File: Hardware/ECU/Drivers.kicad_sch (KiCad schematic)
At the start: 52 parts, among them SW4 SW_DPDT_x2, U10 TC4424A, U5 TC4424A, U6 TC4424A, U7 MC33810, U8 MC33810, U9 TC4424A

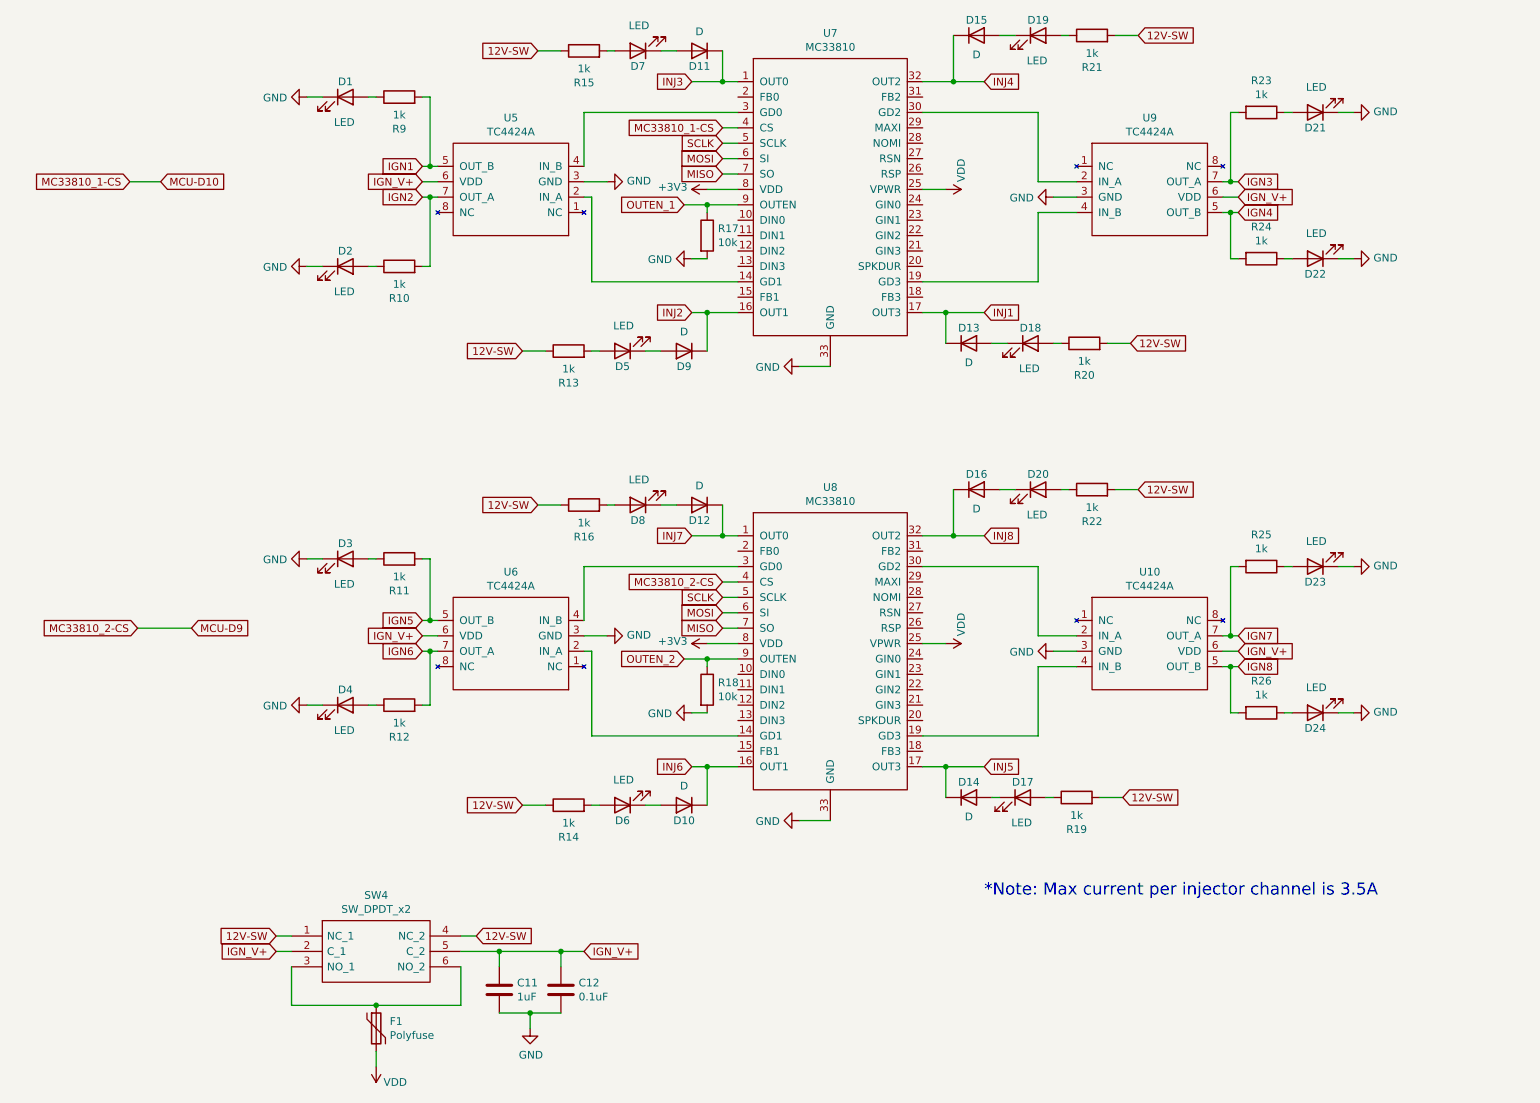
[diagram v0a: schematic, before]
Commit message: PCB
Platine Vernetzt
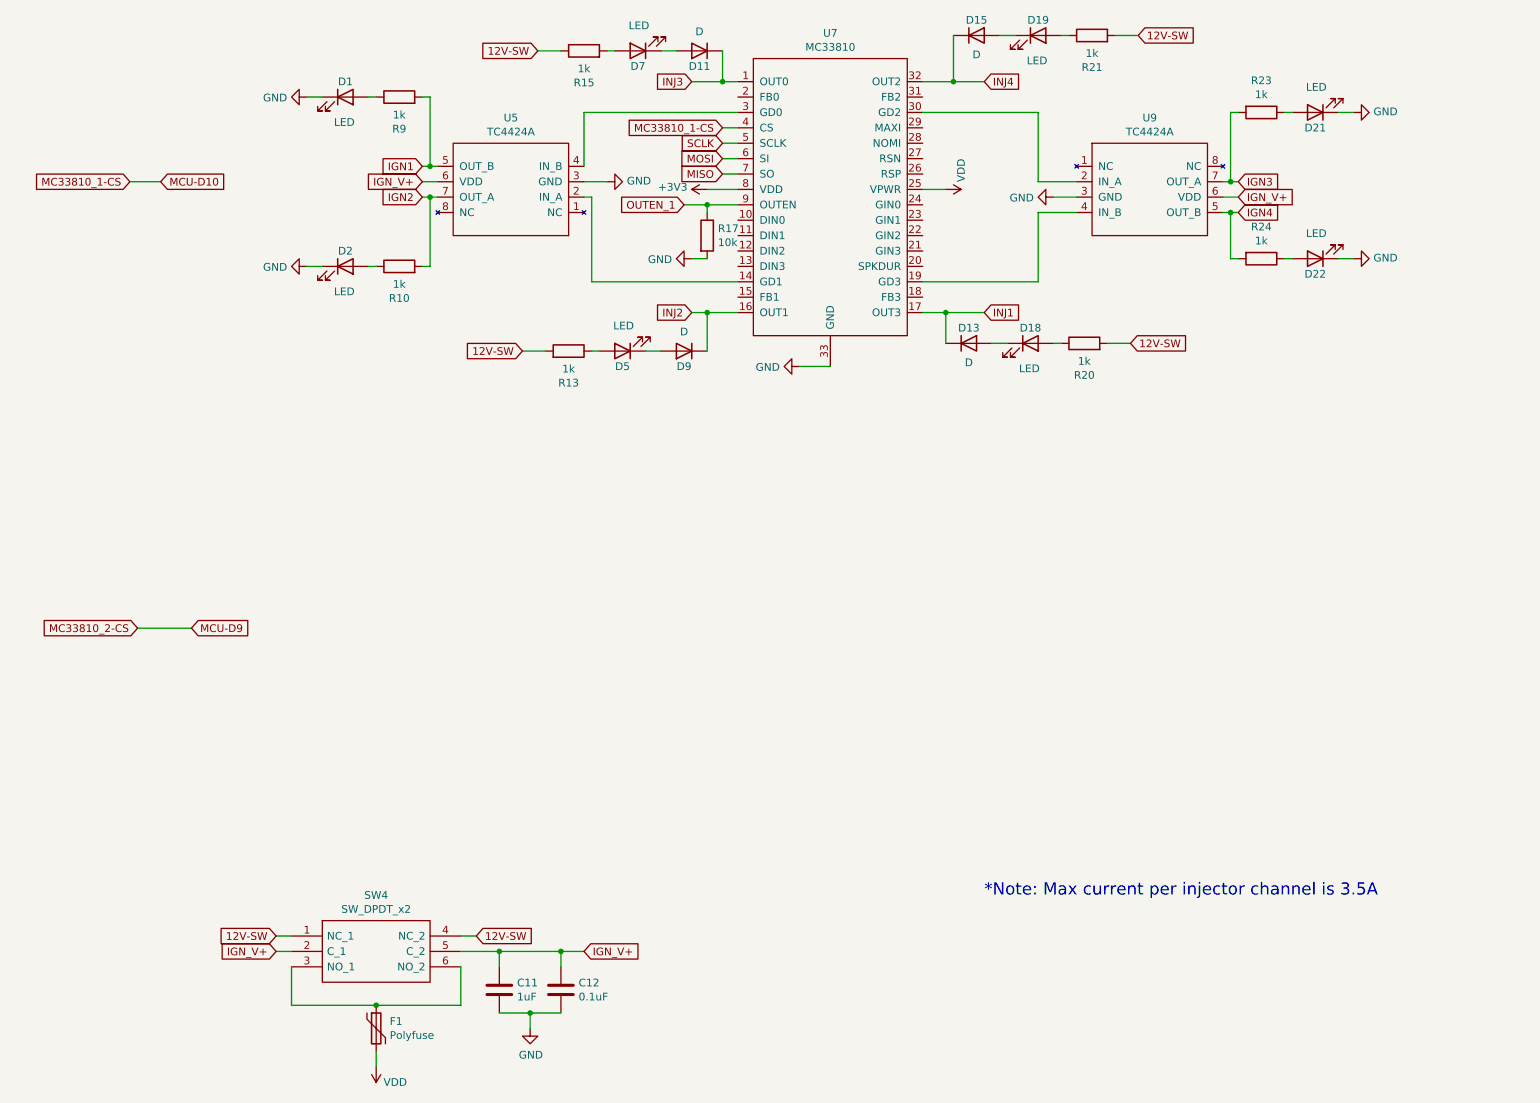
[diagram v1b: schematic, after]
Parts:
- removed D10, D12, D14, D16: D, Diode_SMD:D_SOD-323, symbol Device:D
- removed D17, D20, D23, D24, D3, D4, D6, D8: LED, LED_SMD:LED_0805_2012Metric, symbol Device:LED
- removed R11, R12, R14, R16, R19, R22, R25, R26: 1k, Resistor_SMD:R_0805_2012Metric, symbol Device:R
- removed R18: 10k, Resistor_SMD:R_0805_2012Metric, symbol Device:R
- removed U10, U6: TC4424A, Package_SO:SOIC-8_3.9x4.9mm_P1.27mm, symbol IC_Automotive:TC4424A
- removed U8: MC33810, IC_Automotive:SOIC32-P0.65-33N, symbol IC_Automotive:MC33810
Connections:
- net 12V-SW: now also R13.2; no longer R13.1
- net at D5.2 (A): now also R13.1; no longer R13.2
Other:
- moved on the sheet: R13
